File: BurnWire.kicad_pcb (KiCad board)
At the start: 2 copper layers, 13 parts, among them U1 ADP2303ARDZ

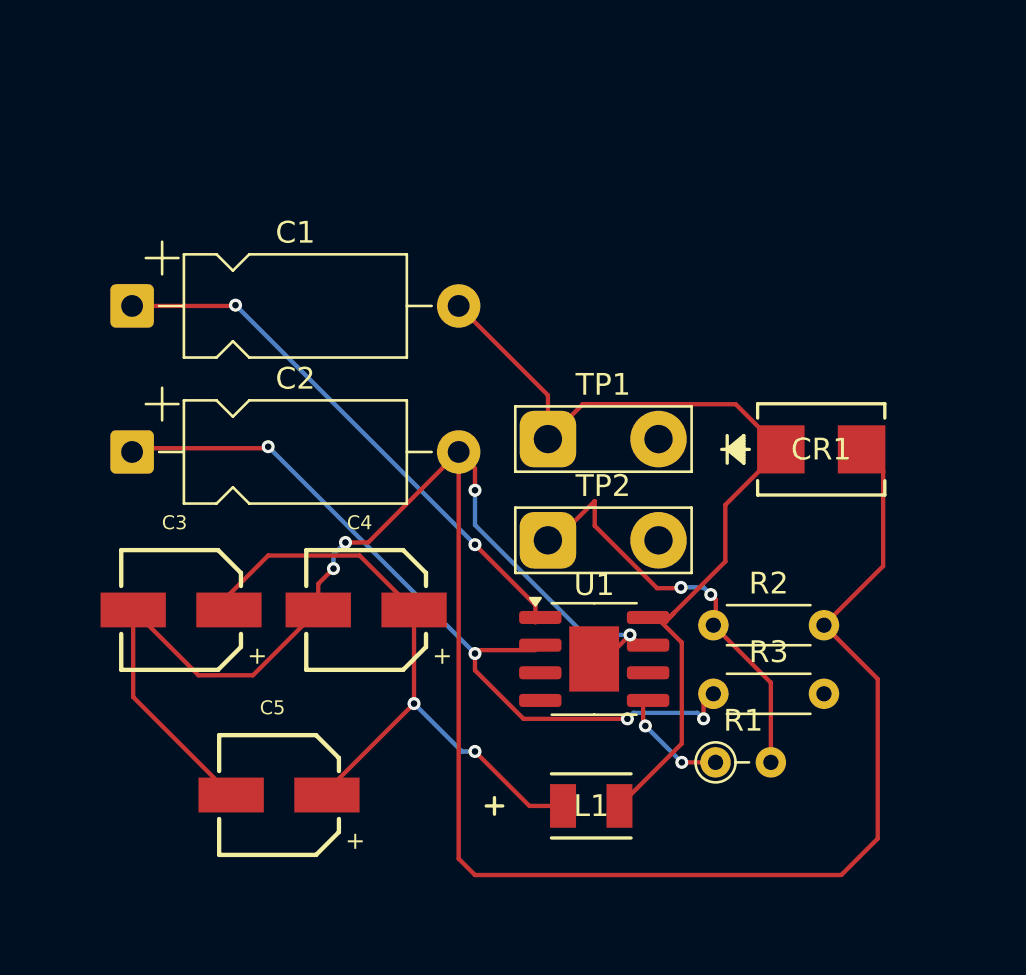
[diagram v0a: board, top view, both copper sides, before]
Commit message: reworked most of the layout
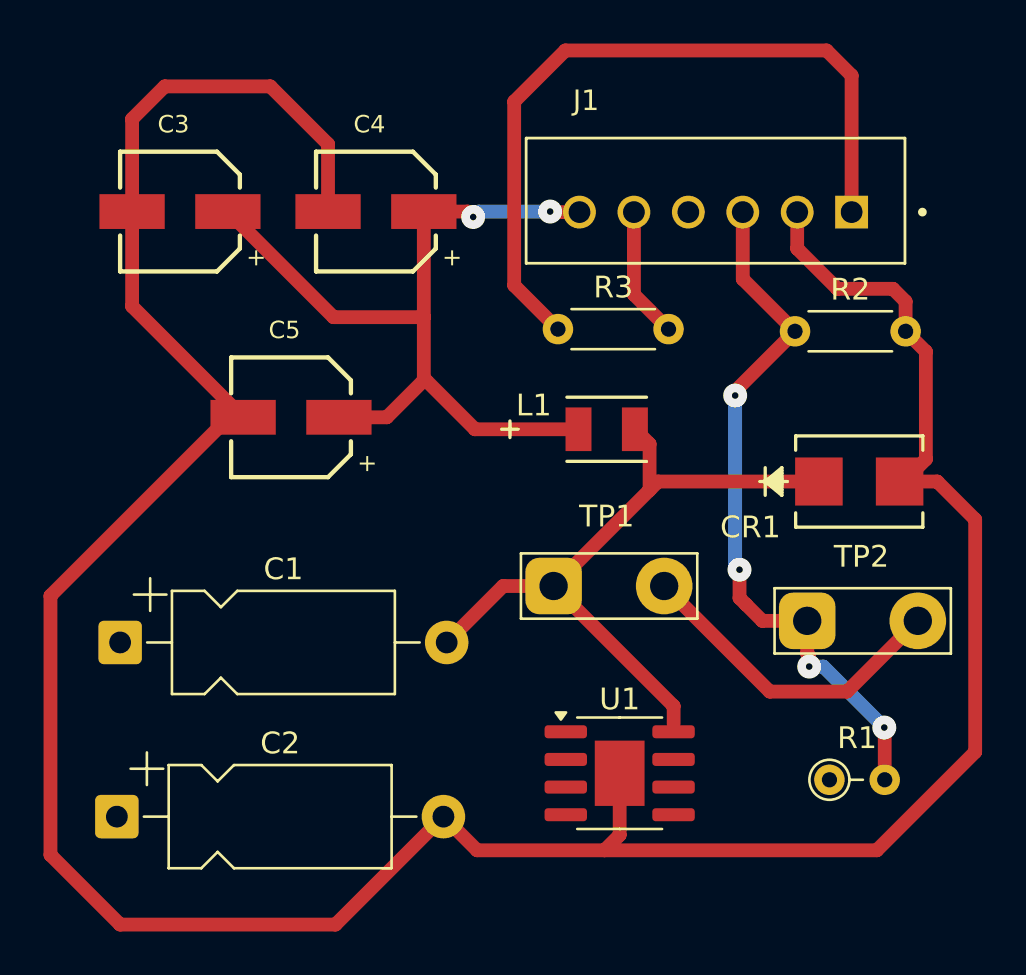
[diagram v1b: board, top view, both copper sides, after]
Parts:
- added J1: B6B-XH-A_LF__SN_, imported_footprints:JST_B6B-XH-A_LF__SN_, F.Cu at (162.1, 80.2)
- moved C4 18.3 mm to (146.4, 80.7)
- moved C3 18.3 mm to (137.4, 80.7)
- moved R3 18.2 mm to (154.8, 86.1)
- moved C5 17.4 mm to (142.6, 90.2)
- moved L1 17.3 mm to (157.1, 90.7)
- moved C2 16.8 mm to (134.6, 108.5)
- moved C1 15.5 mm to (134.7, 100.5)
- moved R2 14.0 mm to (165.7, 86.2)
- moved TP2 12.5 mm to (166.3, 99.5)
- moved TP1 6.76 mm to (154.6, 97.9)
- moved U1 5.38 mm to (157.6, 106.5)
- moved R1 5.29 mm to (167.3, 106.8)
- moved CR1 2.29 mm to (168.7, 93.1)
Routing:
- net GND: track 107.4 -> 137.8 mm, vias 4 -> 0
- net Net-(U1-BST): track 25.0 -> 0.00 mm, vias 2 -> 0
- net (no net): track 0.00 -> 15.0 mm
- net /VCutN: track 19.7 -> 32.2 mm, vias 2 -> 4
- net Net-(U1-SW): track 42.4 -> 31.8 mm
- net /Vout: track 29.9 -> 38.7 mm
- net Net-(U1-PGOOD): track 0.00 -> 6.03 mm
- net Net-(U1-FB): track 4.90 -> 0.00 mm, vias 2 -> 0
- net /VBatt: track 36.3 -> 34.5 mm, vias 4 -> 0
